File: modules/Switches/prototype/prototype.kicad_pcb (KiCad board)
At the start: 6 copper layers, 40.6 x 78.7 mm, 8 parts, among them J1 Conn_01x09, SW1 SW_Push, U1 TL072

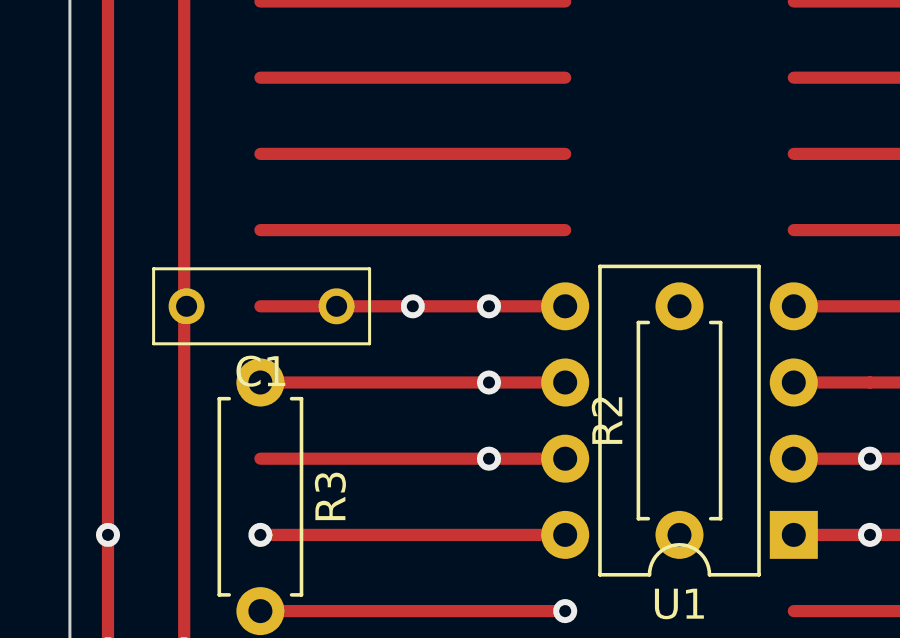
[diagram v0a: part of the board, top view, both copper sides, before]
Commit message: Switches module - prototype wip
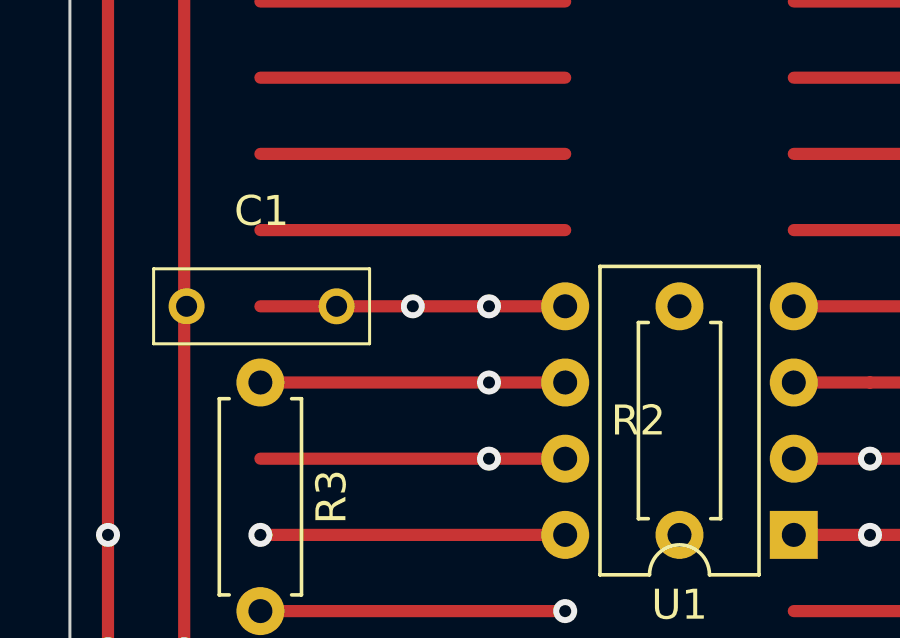
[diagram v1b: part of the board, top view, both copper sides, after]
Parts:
- R3: value R_1K_Output -> 1K
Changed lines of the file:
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@@
     (property "ki_keywords" "R res resistor")
     (attr through_hole)
-    (fp_text reference "R2" (at 3.81 -2.37 90) (layer "F.SilkS")
+    (fp_text reference "R2" (at 3.81 -1.37 180) (layer "F.SilkS")
         (effects (font (size 1 1) (thickness 0.15)))
     )
@@
         (effects (font (size 1 1) (thickness 0.15)))
     )
-    (fp_text value "R_1K_Output" (at 3.81 2.37 -90) (layer "F.Fab")
+    (fp_text value "1K" (at 3.81 2.37 -90) (layer "F.Fab")
         (effects (font (size 1 1) (thickness 0.15)))
     )
@@
     (property "ki_keywords" "cap capacitor film")
     (attr through_hole)
-    (fp_text reference "C1" (at 2.5 -2.2) (layer "F.SilkS")
-        (effects (font (size 1 1) (thickness 0.15)))
-    )
+    (fp_text reference "C1" (at 2.5 3.175) (layer "F.SilkS")
+        (effects (font (size 1 1) (thickness 0.15)))
+    )
